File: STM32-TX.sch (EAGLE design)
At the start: 42 parts, among them IC1 STM32F10XCXT6, Y1 RESONATORSMD

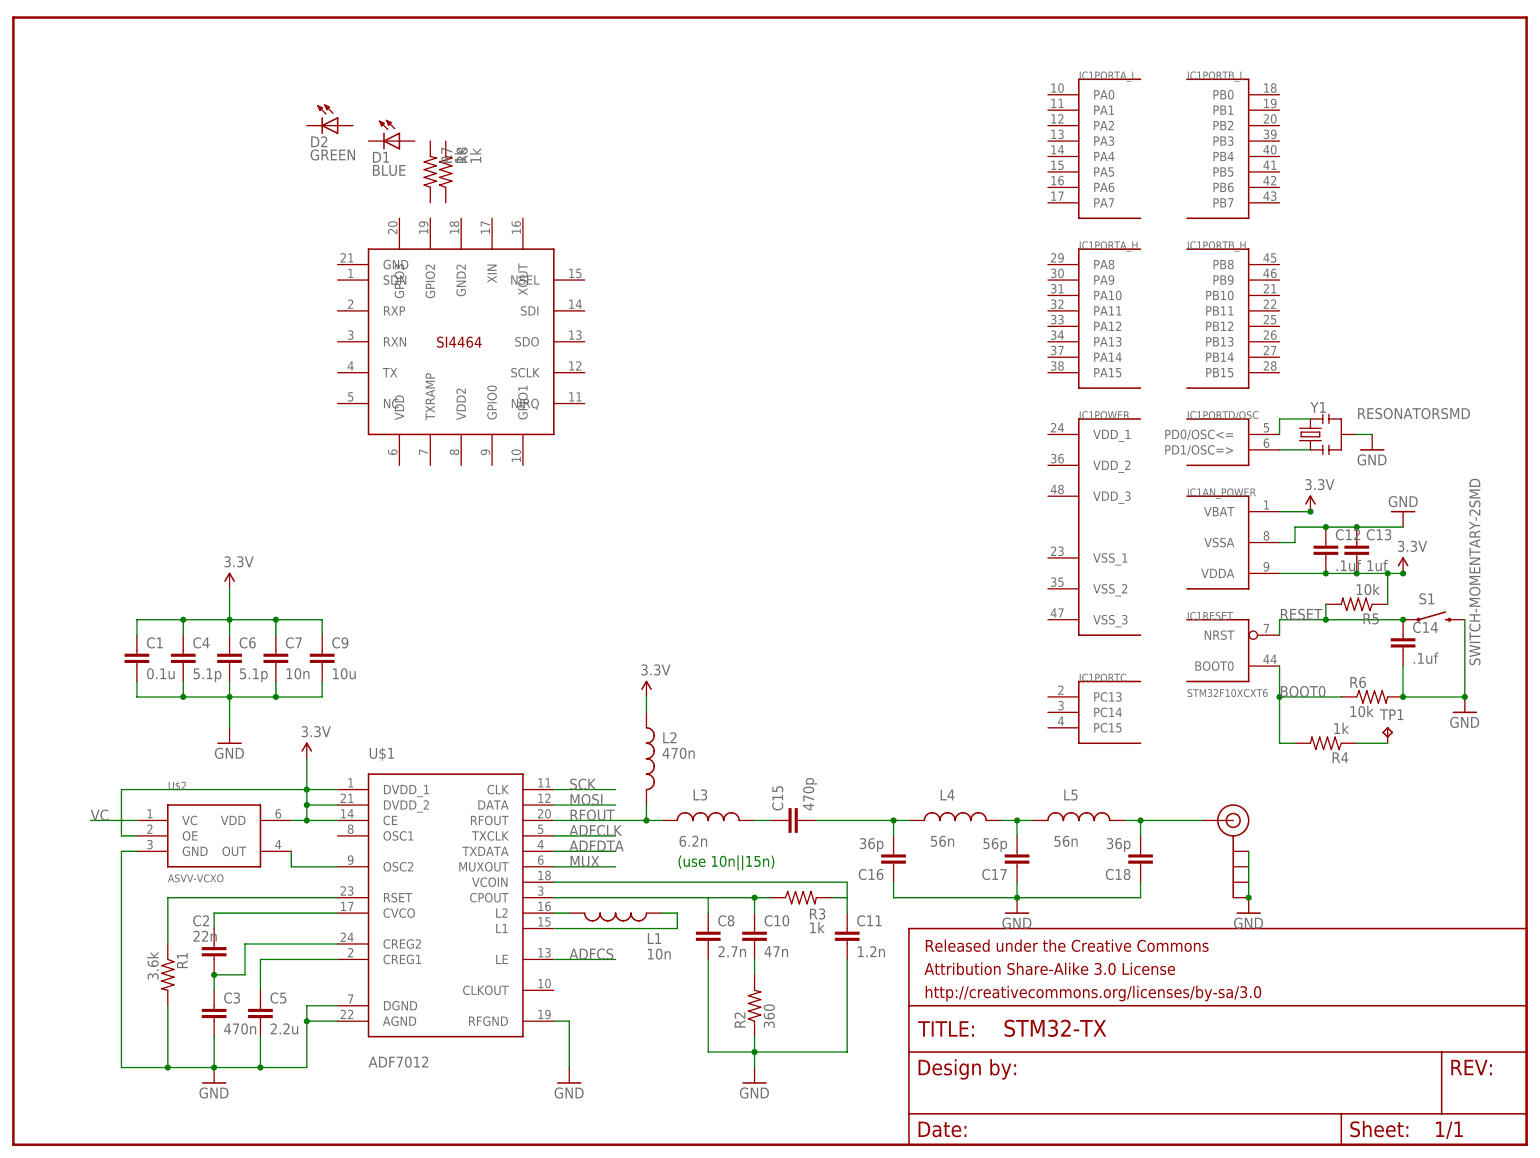
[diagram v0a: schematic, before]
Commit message: work in process
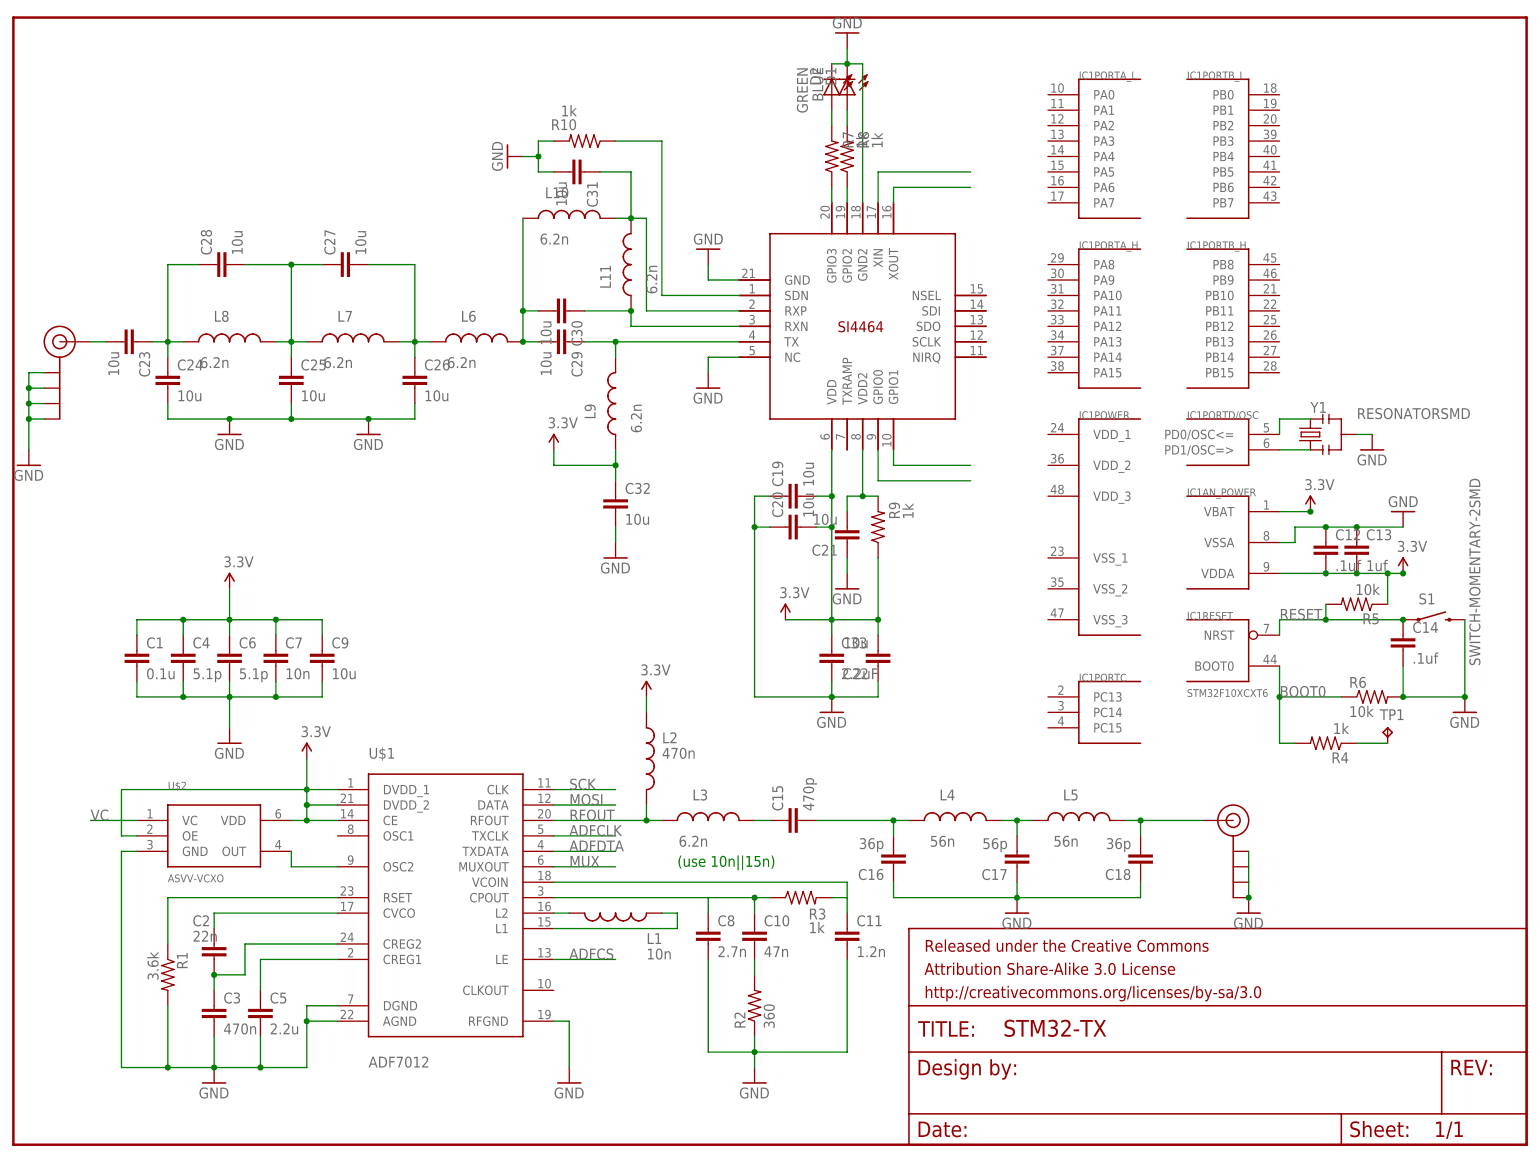
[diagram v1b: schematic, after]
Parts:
- added C19, C20, C21, C22, C23, C24, C25, C26, C27, C28, C29, C30, C31, C32: 10u, SparkFun-Capacitors:CAP0603-CAP
- added C33: 2.2uF, SparkFun-Capacitors:2.2UF-CERCAP-10009
- added J$2: SMA_EDGE, SparkFun-Connectors:SMA_EDGE
- added L10, L11, L6, L7, L8, L9: 6.2n, SparkFun-Passives:INDUCTOR0603
- added R10, R9: 1k, SparkFun-Passives:RESISTOR0603-RES
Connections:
- new net N$18: C23.2, J$2.SIGNAL
- new net N$19: C23.1, C24.1, C28.1, L8.1
- new net N$20: U$3.GPIO1
- new net N$21: C25.1, C27.1, C28.2, L7.1, L8.2
- new net N$22: C26.1, C27.2, L6.1, L7.2
- new net N$23: C29.1, L9.2, U$3.TX
- new net N$24: C29.2, C30.2, L10.1, L6.2
- new net N$25: C30.1, L11.1, U$3.RXN
- new net N$26: C31.1, L10.2, L11.2, U$3.RXP
- new net N$27: R10.1, U$3.SDN
- new net N$31: D1.A, R8.2
- new net N$32: D2.A, R7.2
- new net N$33: R7.1, U$3.GPIO3
- new net N$34: R8.1, U$3.GPIO2
- new net N$35: U$3.XOUT
- new net N$36: U$3.XIN
- new net N$38: U$3.GPIO0
- new net N$39: C21.2, R9.2, U$3.VDD2
- net 3.3V: now also C19.2, C20.2, C22.2, C32.1, C33.1, L9.1, R9.1, U$3.VDD
- net GND: now also C19.1, C20.1, C21.1, C22.1, C24.2, C25.2, C26.2, C31.2, C32.2, C33.2, D1.C, D2.C, J$2.GND@0, J$2.GND@1, J$2.GND@2, J$2.GND@3, R10.2, U$3.GND, U$3.GND2, U$3.NC 
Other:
- moved on the sheet: D1, D2, R7, R8
